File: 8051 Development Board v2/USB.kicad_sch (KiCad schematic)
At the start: 10 parts, among them J7 USB4730-GF-A, U16 USBLC6-2SC6, U17 CP2102N-Axx-xQFN20

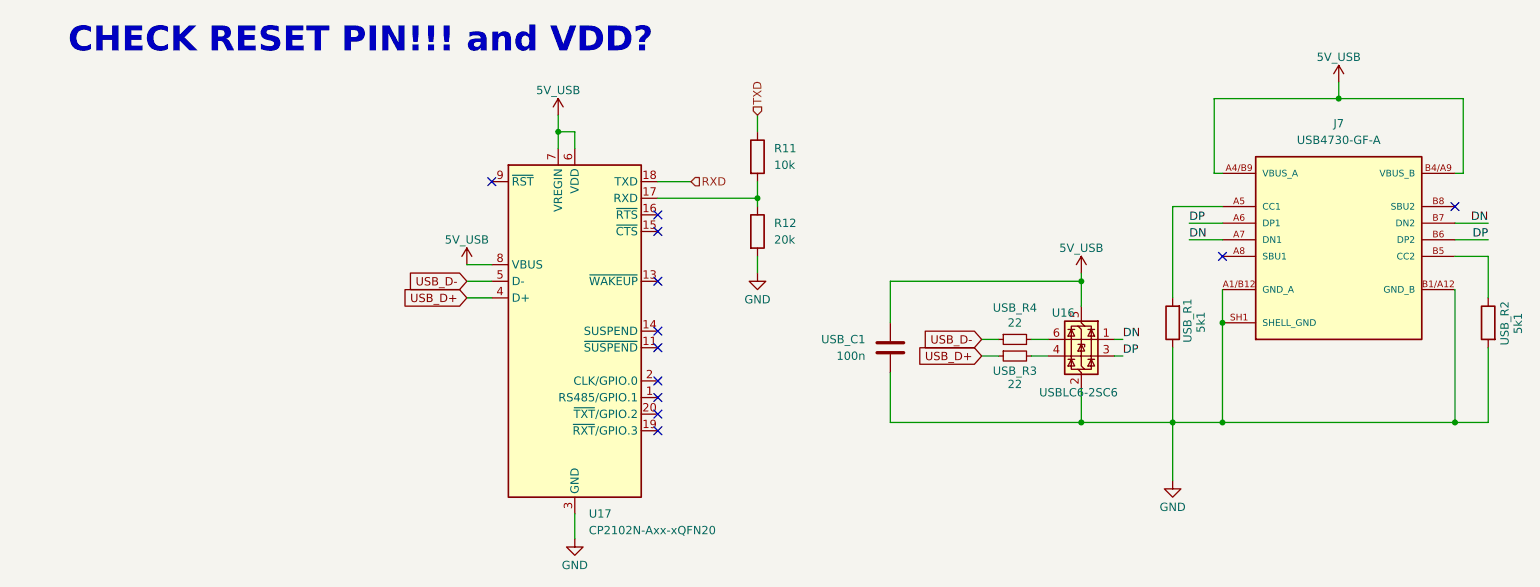
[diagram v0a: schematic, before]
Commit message: usb
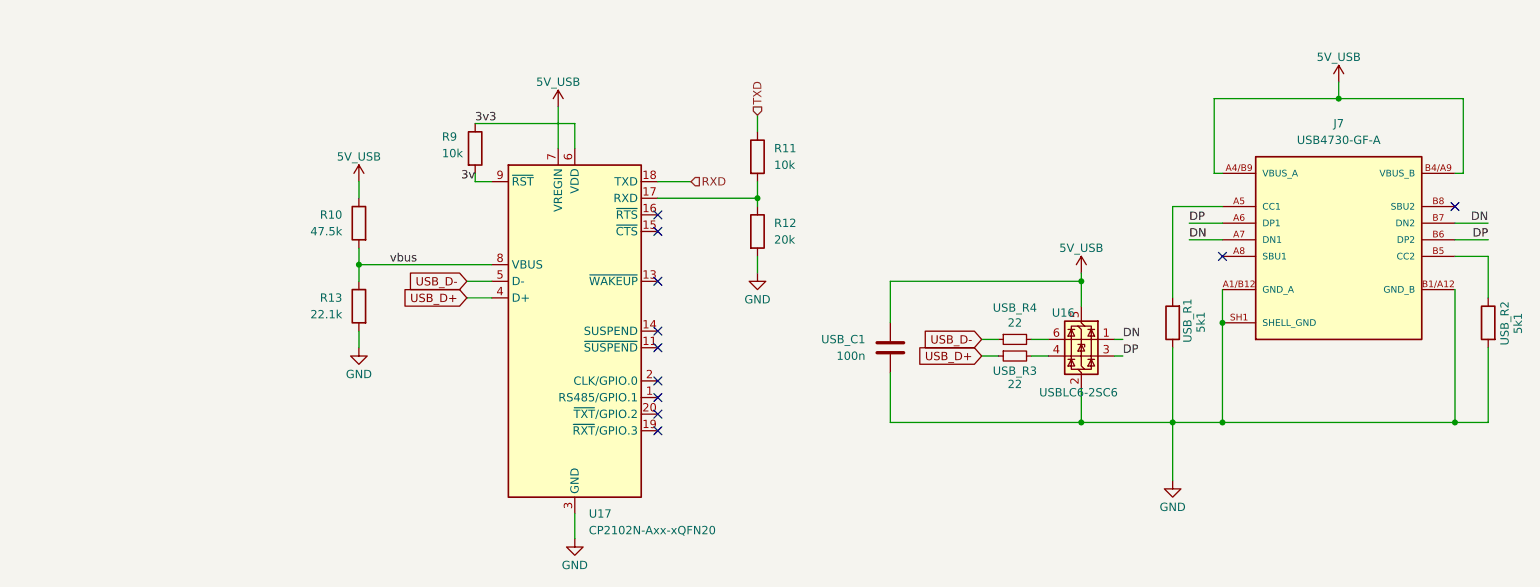
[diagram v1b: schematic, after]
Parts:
- added R10: 47.5k, Resistor_SMD:R_1206_3216Metric, symbol Device:R
- added R13: 22.1k, Resistor_SMD:R_1206_3216Metric, symbol Device:R
- added R9: 10k, Resistor_SMD:R_1206_3216Metric, symbol Device:R
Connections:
- net 5V_USB: now also R10.1; no longer U17.6 (VDD), U17.8 (VBUS)
- net GND: now also R13.2
- net 3v: now reaches U17.9 (~{RST})
- net 3v: now also R9.2
- new net 3v3: R9.1, U17.6 (VDD)
- new net vbus: R10.2, R13.1, U17.8 (VBUS)
- no-connect marks 12 -> 11
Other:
- note removed: "CHECK RESET PIN!!! and VDD?"
